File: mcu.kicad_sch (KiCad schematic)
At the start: 10 parts, among them J1 Conn_01x05_Socket, U1 ATSAMD21G18A-A

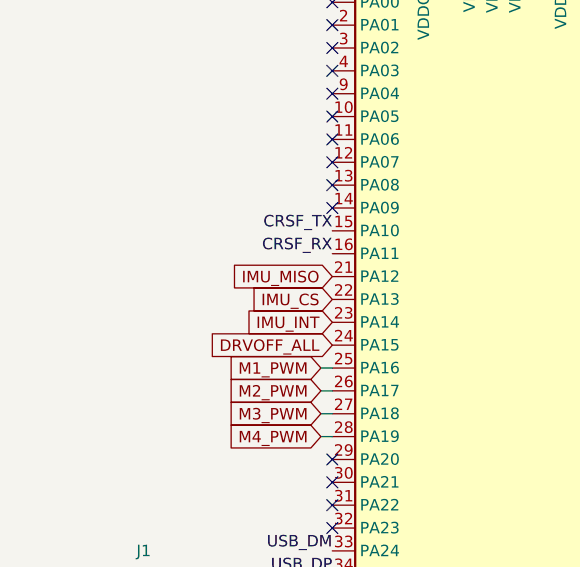
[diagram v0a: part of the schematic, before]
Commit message: done?
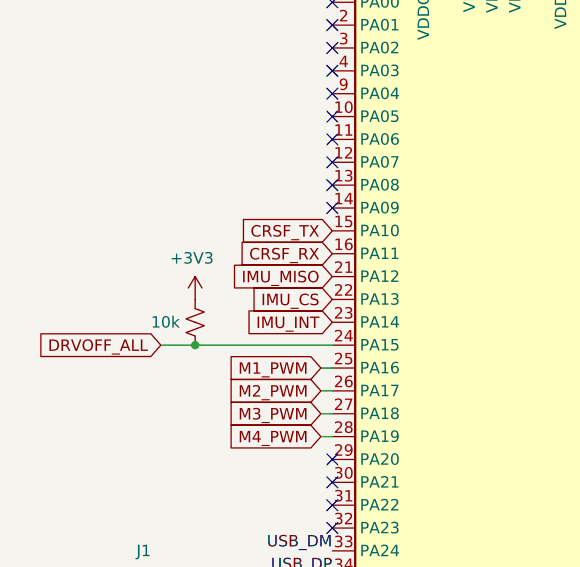
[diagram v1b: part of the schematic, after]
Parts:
- added R4: 10k, Resistor_SMD:R_0402_1005Metric_Pad0.72x0.64mm_HandSolder, symbol Device:R_Small_US
- J1: footprint Connector_PinHeader_2.54mm:PinHeader_1x05_P2.54mm_Vertical -> Connector_PinSocket_1.00mm:PinSocket_1x05_P1.00mm_Vertical_SMD_Pin1Left
- R1, R2: footprint Resistor_SMD:R_0603_1608Metric_Pad0.98x0.95mm_HandSolder -> Resistor_SMD:R_0402_1005Metric_Pad0.72x0.64mm_HandSolder
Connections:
- net +3V3: now also R4.2
- net DRVOFF_ALL: now also R4.1
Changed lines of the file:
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@@
+	)
+	(junction
+		(at 80.01 130.81)
+		(diameter 0)
+		(color 0 0 0 0)
 	)
 	(junction
@@
 	(wire
 		(pts
+			(xy 80.01 130.81) (xy 95.25 130.81)
+		)
+		(stroke
+			(width 0)
+			(type default)
+		)
+	)
+	(wire
+		(pts
 			(xy 115.57 181.61) (xy 114.3 181.61)
 		)
@@
 		)
 	)
-	(label "CRSF_RX"
-		(at 95.25 120.65 180)
-		(effects
-			(font
-				(size 1.27 1.27)
-			)
-			(justify right bottom)
-		)
-	)
-	(label "CRSF_TX"
-		(at 95.25 118.11 180)
-		(effects
-			(font
-				(size 1.27 1.27)
-			)
-			(justify right bottom)
+	(wire
+		(pts
+			(xy 76.2 130.81) (xy 80.01 130.81)
+		)
+		(stroke
+			(width 0)
+			(type default)
 		)
 	)
@@
 		)
 	)
+	(global_label "CRSF_RX"
+		(shape input)
+		(at 95.25 120.65 180)
+		(fields_autoplaced yes)
+		(effects
+			(font
+				(size 1.27 1.27)
+			)
+			(justify right)
+		)
+		(property "Intersheetrefs" "${INTERSHEET_REFS}"
+			(at 83.9796 120.65 0)
+			(effects
+				(font
+					(size 1.27 1.27)
+				)
+				(justify right)
+				(hide yes)
+			)
+		)
+	)
 	(global_label "IMU_SCK"
 		(shape input)
@@
 		)
 	)
-	(global_label "DRVOFF_ALL"
+	(global_label "CRSF_TX"
 		(shape input)
-		(at 95.25 130.81 180)
+		(at 95.25 118.11 180)
 		(fields_autoplaced yes)
 		(effects
@@
 		)
 		(property "Intersheetrefs" "${INTERSHEET_REFS}"
-			(at 81.0161 130.81 0)
+			(at 84.282 118.11 0)
+			(effects
+				(font
+					(size 1.27 1.27)
+				)
+				(justify right)
+				(hide yes)
+			)
+		)
+	)
+	(global_label "DRVOFF_ALL"
+		(shape input)
+		(at 76.2 130.81 180)
+		(fields_autoplaced yes)
+		(effects
+			(font
+				(size 1.27 1.27)
+			)
+			(justify right)
+		)
+		(property "Intersheetrefs" "${INTERSHEET_REFS}"
+			(at 61.9661 130.81 0)
 			(effects
 				(font
@@
 		(on_board yes)
 		(dnp no)
-		(fields_autoplaced yes)
 		(property "Reference" "R2"
 			(at 83.82 160.02 90)
@@
 			)
 		)
-		(property "Footprint" "Resistor_SMD:R_0603_1608Metric_Pad0.98x0.95mm_HandSolder"
+		(property "Footprint" "Resistor_SMD:R_0402_1005Metric_Pad0.72x0.64mm_HandSolder"
 			(at 83.82 166.37 0)
 			(effects
@@
 			)
 		)
-		(property "Datasheet" "~"
+		(property "Datasheet" ""
 			(at 83.82 166.37 0)
 			(effects
@@
 			)
 		)
-		(property "Description" "Resistor, small US symbol"
+		(property "Description" ""
 			(at 83.82 166.37 0)
 			(effects
@@
 	)
 	(symbol
+		(lib_id "Device:R_Small_US")
+		(at 80.01 128.27 180)
+		(unit 1)
+		(exclude_from_sim no)
+		(in_bom yes)
+		(on_board yes)
+		(dnp no)
+		(property "Reference" "R4"
+			(at 73.66 128.27 90)
+			(effects
+				(font
+					(size 1.27 1.27)
+				)
+				(hide yes)
+			)
+		)
+		(property "Value" "10k"
+			(at 76.708 128.27 0)
+			(effects
+				(font
+					(size 1.27 1.27)
+				)
+			)
+		)
+		(property "Footprint" "Resistor_SMD:R_0402_1005Metric_Pad0.72x0.64mm_HandSolder"
+			(at 80.01 128.27 0)
+			(effects
+				(font
+					(size 1.27 1.27)
+				)
+				(hide yes)
+			)
+		)
+		(property "Datasheet" ""
+			(at 80.01 128.27 0)
+			(effects
+				(font
+					(size 1.27 1.27)
+				)
+				(hide yes)
+			)
+		)
+		(property "Description" ""
+			(at 80.01 128.27 0)
+			(effects
+				(font
+					(size 1.27 1.27)
+				)
+				(hide yes)
+			)
+		)
+		(pin "2"
+		)
+		(pin "1"
+		)
+		(instances
+			(project "neodrone-v1"
+				(path "/ec430d83-72cd-4950-a197-fb5338d7c552/91a2a763-470d-4a4d-9e8e-b9069d2f4064"
+					(reference "R4")
+					(unit 1)
+				)
+			)
+		)
+	)
+	(symbol
 		(lib_id "power:GND")
 		(at 125.73 85.09 90)
@@
 			)
 		)
-		(property "Footprint" "Connector_PinHeader_2.54mm:PinHeader_1x05_P2.54mm_Vertical"
+		(property "Footprint" "Connector_PinSocket_1.00mm:PinSocket_1x05_P1.00mm_Vertical_SMD_Pin1Left"
 			(at 73.66 163.83 0)
 			(effects
@@
 			)
 		)
-		(property "Footprint" "Resistor_SMD:R_0603_1608Metric_Pad0.98x0.95mm_HandSolder"
+		(property "Footprint" "Resistor_SMD:R_0402_1005Metric_Pad0.72x0.64mm_HandSolder"
 			(at 87.63 176.53 0)
 			(effects
@@
 			)
 		)
-		(property "Datasheet" "~"
+		(property "Datasheet" ""
 			(at 87.63 176.53 0)
 			(effects
@@
 			)
 		)
-		(property "Description" "Resistor, small US symbol"
+		(property "Description" ""
 			(at 87.63 176.53 0)
 			(effects
@@
 					(unit 1)
 				)
+			)
+		)
+	)
+	(symbol
+		(lib_id "power:+3V3")
+		(at 80.01 125.73 0)
+		(unit 1)
+		(exclude_from_sim no)
+		(in_bom yes)
+		(on_board yes)
+		(dnp no)
+		(property "Reference" "#PWR012"
+			(at 80.01 129.54 0)
+			(effects
+				(font
+					(size 1.27 1.27)
+				)
+				(hide yes)
+			)
+		)
+		(property "Value" "+3V3"
+			(at 77.216 121.158 0)
+			(effects
+				(font
+					(size 1.27 1.27)
+				)
+				(justify left)
+			)
+		)
+		(property "Footprint" ""
+			(at 80.01 125.73 0)
+			(effects
+				(font
+					(size 1.27 1.27)
+				)
+				(hide yes)
+			)
+		)
+		(property "Datasheet" ""
+			(at 80.01 125.73 0)
+			(effects
+				(font
+					(size 1.27 1.27)
+				)
+				(hide yes)
+			)
+		)
+		(property "Description" "Power symbol creates a global label with name \"+3V3\""
+			(at 80.01 125.73 0)
+			(effects
+				(font
+					(size 1.27 1.27)
+				)
+				(hide yes)
+			)
+		)
+		(pin "1"
+		)
+		(instances
+			(project "neodrone-v1"
+				(path "/ec430d83-72cd-4950-a197-fb5338d7c552/91a2a763-470d-4a4d-9e8e-b9069d2f4064"
+					(reference "#PWR012")
+					(unit 1)
+				)
